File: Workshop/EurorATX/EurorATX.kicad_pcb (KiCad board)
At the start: 2 copper layers, 82.6 x 130.8 mm, 51 parts, among them J1 FRONT PANEL MAGIC, J14 USB C PD IN, J15 EURO CH 2, J16 MAINBOARD MAGIC, J17 EURO BUS, J18 EURO BUS, J19 EURO CH 1, J20 EURO BUS, J21 EURO BUS, J22 EURO BUS, J23 EURO BUS, J24 EURO BUS, J25 EURO BUS, J26 EURO BUS, J27 EURO BUS, J28 EURO BUS, J29 EURO BUS, U2 30 Watt Rail 2, U3 CH224K, U4 30W Rail 1

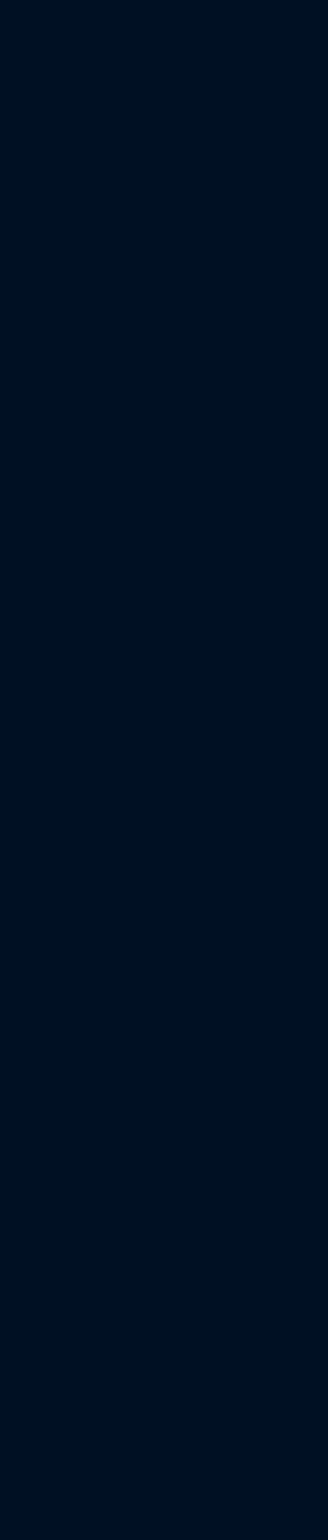
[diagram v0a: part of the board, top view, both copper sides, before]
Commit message: polished and PSU, did a todo, much ado about something
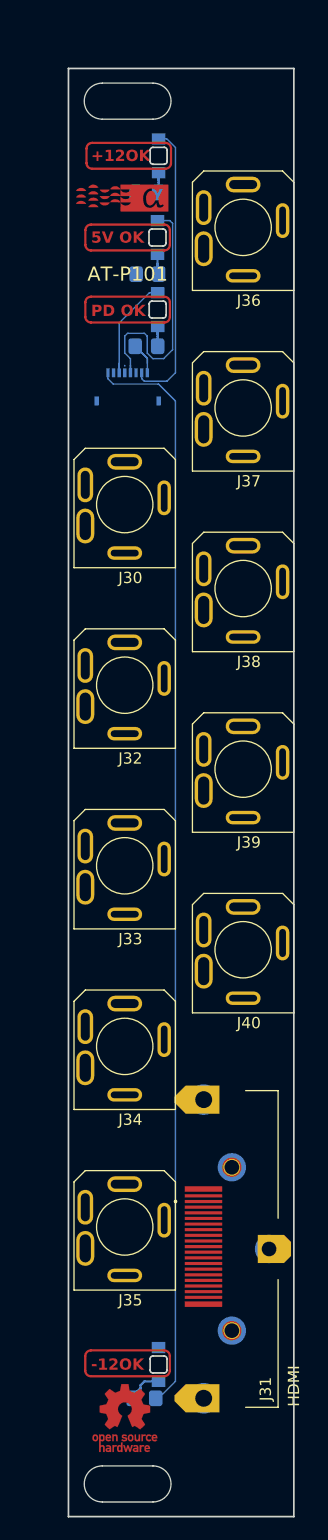
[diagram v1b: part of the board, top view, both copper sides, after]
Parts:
- added D1: LED (Red), AT-Footprints:WL-SMRD_1205, F.Cu at (262.4, 43.9)
- added D2: LED (Yellow), AT-Footprints:WL-SMRD_1205, F.Cu at (262.3, 51.1)
- added D3: LED (Green), AT-Footprints:WL-SMRD_1205, F.Cu at (262.3, 57.5)
- added D4: LED (Blue), AT-Footprints:WL-SMRD_1205, F.Cu at (262.4, 151.1)
- added GFX2: FRONT PANEL OSHW, Symbol:OSHW-Logo_5.7x6mm_Copper, F.Cu at (259.4, 155.8)
- added GFX3: FRONT PANEL AT LOGO, AT-Footprints:at-logo-ex-cu, F.Cu at (259.2, 47.0)
- added J1: FRONT PANEL MAGIC, AT-Footprints:AMPHENOL_F33B-1A7Q1-E8C08, B.Cu at (259.6, 64.8)
- added J30: AudioJack3_SwitchT, AT-Footprints:SJ3-3505, F.Cu at (259.4, 74.8)
- added J31: HDMI, AT-Footprints:AMPHENOL_10078837-001LF, F.Cu at (268.9, 140.8)
- added J32: AudioJack3_SwitchT, AT-Footprints:SJ3-3505, F.Cu at (259.4, 90.8)
- added J33: AudioJack3_SwitchT, AT-Footprints:SJ3-3505, F.Cu at (259.4, 106.8)
- added J34: AudioJack3_SwitchT, AT-Footprints:SJ3-3505, F.Cu at (259.4, 122.9)
- added J35: AudioJack3_SwitchT, AT-Footprints:SJ3-3505, F.Cu at (259.4, 138.9)
- added J36: AudioJack3_SwitchT, AT-Footprints:SJ3-3505, F.Cu at (269.9, 50.2)
- added J37: AudioJack3_SwitchT, AT-Footprints:SJ3-3505, F.Cu at (269.9, 66.2)
- added J38: AudioJack3_SwitchT, AT-Footprints:SJ3-3505, F.Cu at (269.9, 82.2)
- added J39: AudioJack3_SwitchT, AT-Footprints:SJ3-3505, F.Cu at (269.9, 98.3)
- added J40: AudioJack3_SwitchT, AT-Footprints:SJ3-3505, F.Cu at (269.9, 114.3)
- added R1: 500R, Resistor_SMD:R_0805_2012Metric_Pad1.20x1.40mm_HandSolder, B.Cu at (261.4, 47.1)
- added R2: 150R, Resistor_SMD:R_0805_2012Metric_Pad1.20x1.40mm_HandSolder, B.Cu at (261.4, 54.4)
- added R3: 500, Resistor_SMD:R_0805_2012Metric_Pad1.20x1.40mm_HandSolder, B.Cu at (261.3, 60.7)
- added R4: 500, Resistor_SMD:R_0805_2012Metric_Pad1.20x1.40mm_HandSolder, B.Cu at (261.1, 154.1)
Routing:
- net LED BLU: track 96.7 -> 193.4 mm
- net LED RED: track 26.0 -> 52.0 mm
- net LED YLW: track 23.3 -> 46.6 mm
- net LED GRN: track 9.77 -> 19.5 mm
- net FP GND: track 6.07 -> 12.1 mm
- net Net-(D4-K): track 3.41 -> 6.83 mm
- net Net-(D2-K): track 2.24 -> 4.48 mm
- net Net-(D1-K): track 1.97 -> 3.94 mm
- net Net-(D3-K): track 1.97 -> 3.94 mm
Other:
- board size 82.6 x 130.8 mm -> 167.6 x 133.3 mm
